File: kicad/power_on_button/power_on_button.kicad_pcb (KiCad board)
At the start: 2 copper layers, 23.2 x 24.1 mm, 6 parts, among them J1 Conn_01x02_Pin, SW1 B3W-1000

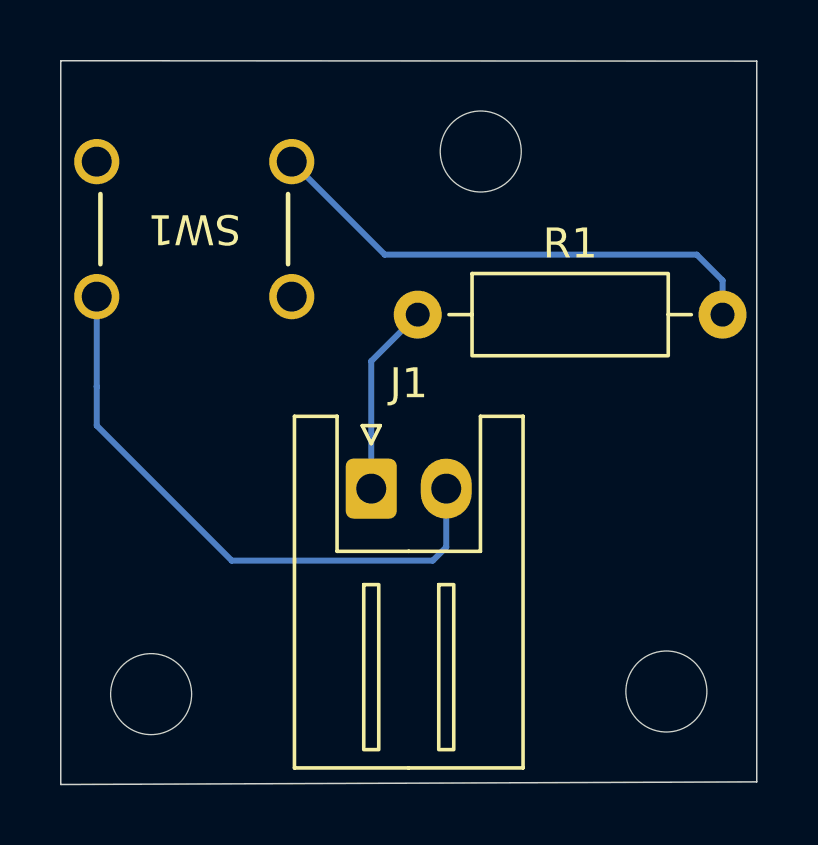
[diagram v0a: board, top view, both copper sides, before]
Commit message: wip
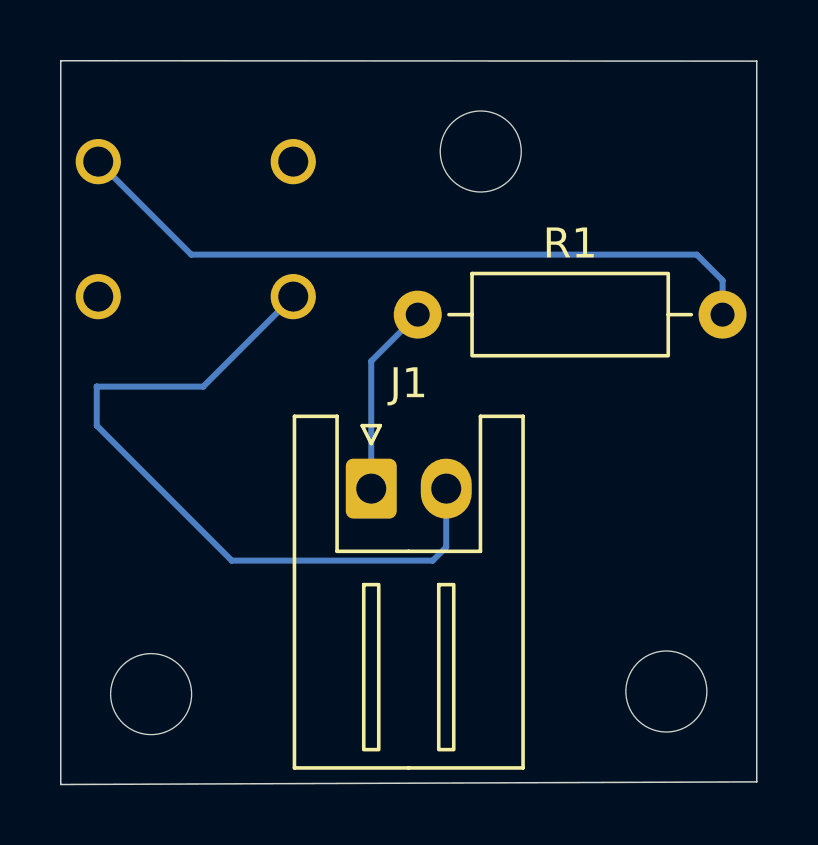
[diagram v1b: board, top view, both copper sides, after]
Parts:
- SW1: moved to B.Cu
- moved SW1 6.45 mm to (220.6, 107.5), turned to 0 degrees
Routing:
- net Net-(R1-Pad2): track 17.1 -> 23.6 mm
- net /Btn1: track 20.0 -> 24.7 mm
